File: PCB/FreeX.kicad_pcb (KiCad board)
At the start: 2 copper layers, 2 parts, among them U1 W25Q32JVZPIQ, U3 ESP32-D0WDQ6

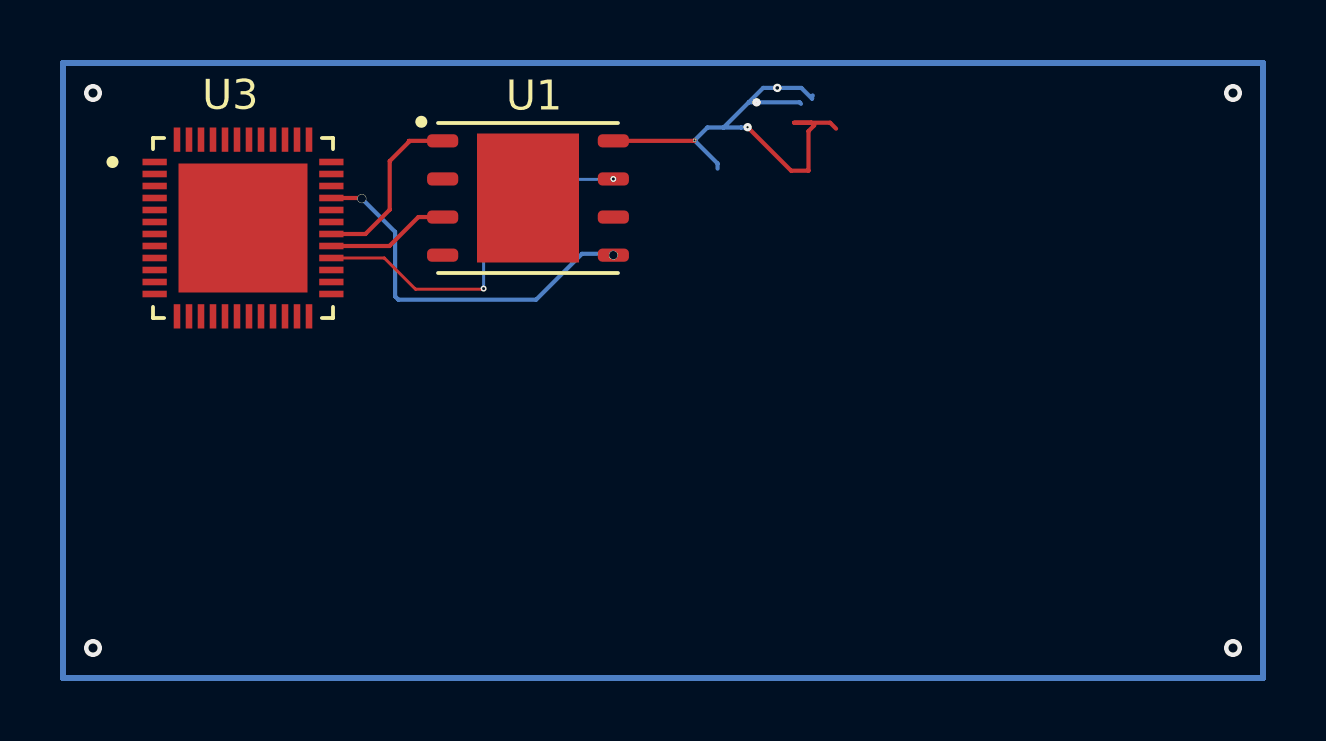
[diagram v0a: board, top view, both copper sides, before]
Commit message: 9th, March 2025
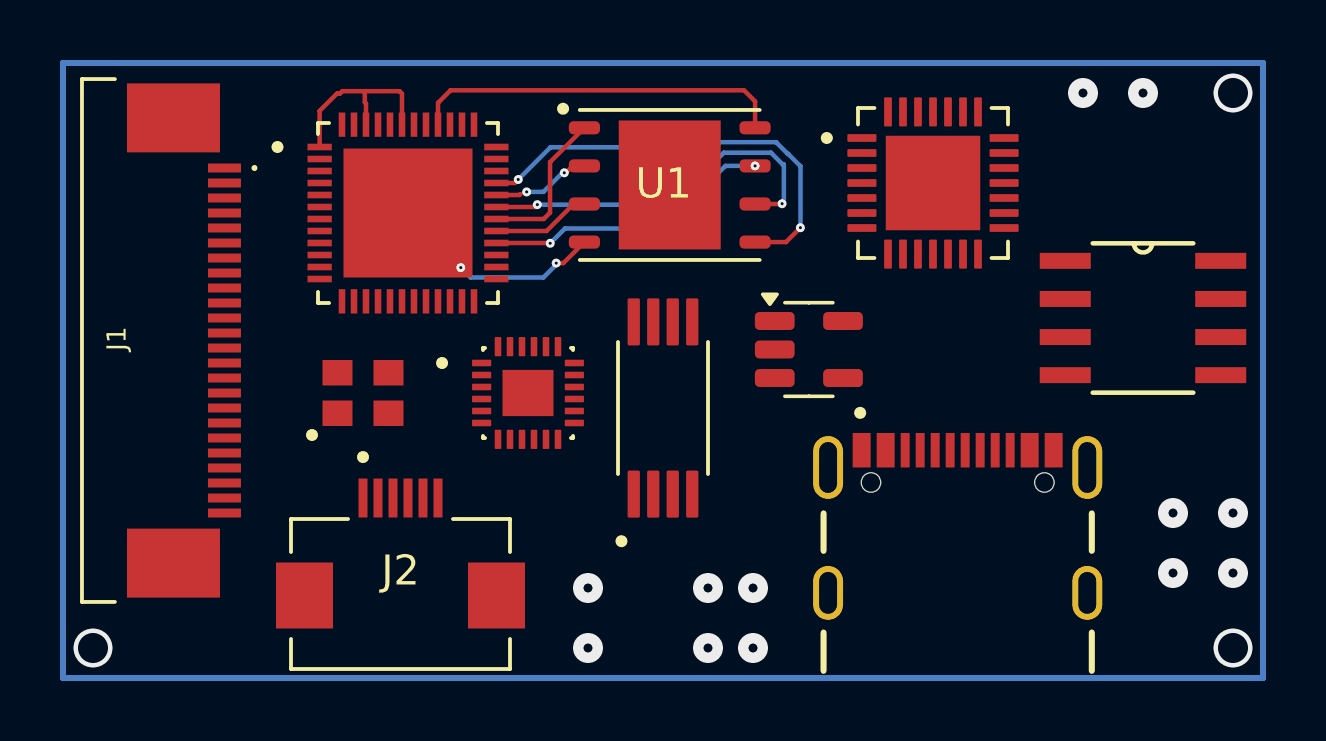
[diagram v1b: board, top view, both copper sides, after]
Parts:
- added J1: 2-1734839-4, 2-1734839-4 pin-24:2-1734839-4 pin-24, F.Cu at (116.7, 89.8)
- added J2: TF31-6S-0.5SH_800_, TF31-6S-0.5SH_800-6-pins:TF31-6S-0.5SH_800-6-pins, F.Cu at (124.2, 98.2)
- added J3: USB4105-GF-A, USB4105-GF-A TYPE C:USB4105-GF-A TYPE C, F.Cu at (142.8, 98.2)
- added U2: MPU-9250, MPU-9250 SENSOR:MPU-9250 SENSOR, F.Cu at (128.5, 91.5)
- added U4: CP2102, CP2102_USB-to-Serial:CP2102_USB-to-Serial, F.Cu at (142.0, 84.5)
- added U5: TC2014-3.3VxCTTR, Package_TO_SOT_SMD:SOT-23-5, F.Cu at (137.9, 90.0)
- added U6: LM358PW, LM358PW-Amplifier:LM358PW-Amplifier, F.Cu at (133.0, 92.0)
- added U7: TDA7052AT_N2, TDA7052AT_N2-Amplifier:TDA7052AT_N2-Amplifier, F.Cu at (149.0, 89.0)
- added Y1: WE-SPXO_IQXO-791, STP_831056298-Crystal-Oscillator:STP_831056298-Crystal-Oscillator, F.Cu at (123.0, 91.5)
- moved U3 5.52 mm to (124.5, 85.5)
- moved U1 4.74 mm to (133.2, 84.6)
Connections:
- U1 pad 8: VDD SDIO -> /VDD SDIO
- U3 pad 40: unconnected-(U3-U0RXD-Pad40) -> /VDD SDIO
- U3 pad 49: unconnected-(U3-GND-Pad49) -> GND
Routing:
- net VDD SDIO: track 17.9 -> 0.00 mm, vias 4 -> 0
- net Net-(U1-CLK): track 0.00 -> 12.7 mm, vias 0 -> 2
- net /VDD SDIO: track 0.00 -> 12.5 mm
- net Net-(U3-VDDA-Pad1): track 0.00 -> 6.42 mm
- net GND: track 0.00 -> 4.77 mm, vias 0 -> 2
- net Net-(U1-DO(IO1)): track 0.00 -> 3.11 mm, vias 0 -> 2
- net Net-(U1-~{HOLD}/RESET(IO3)): track 12.0 -> 9.70 mm
- net Net-(U1-DI(IO0)): track 12.7 -> 14.8 mm, vias 2 -> 15
- net Net-(U1-~{CS}): track 6.41 -> 5.18 mm
- net Net-(U1-~{WP}(IO2)): track 4.11 -> 3.31 mm
- net unconnected-(U7-OUT--Pad8): vias 0 -> 1
- net (no net): vias 4 -> 1
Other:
- board text added: "+"
- board text added: "Buzzer L"
- board text added: "Buzzer R"
- board text added: "Distance L"
- board text added: "Distance R"
- board text added: "MIC"
- board text added: "Speaker"

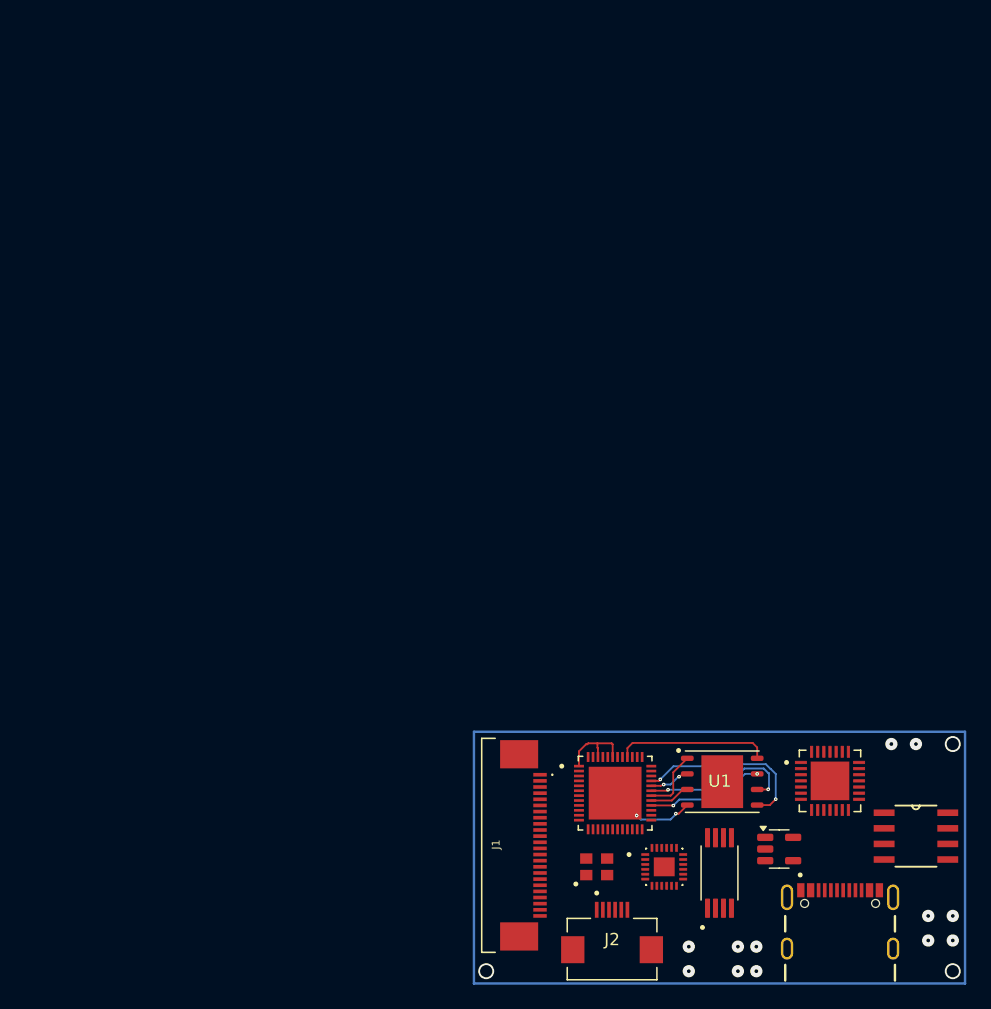
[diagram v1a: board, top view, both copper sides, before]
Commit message: 14th, march. 2025
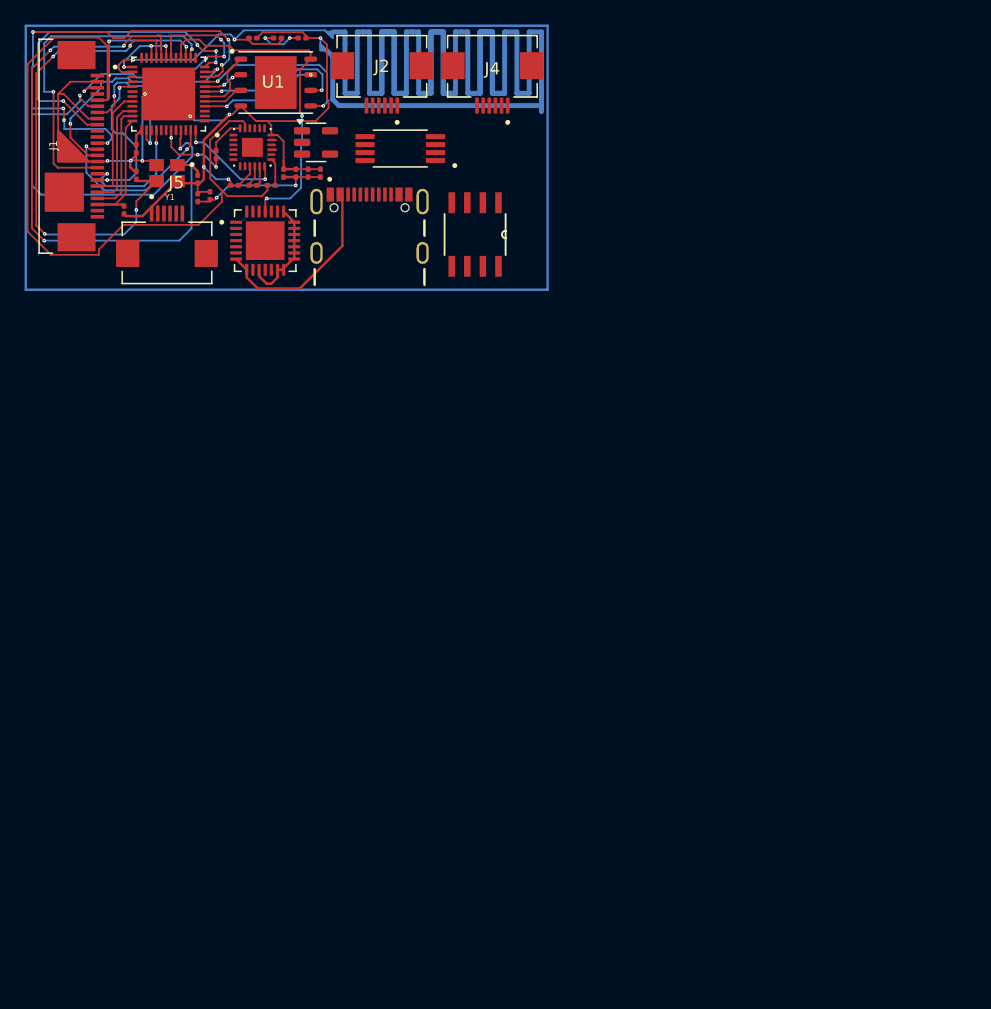
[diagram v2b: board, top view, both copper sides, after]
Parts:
- added C1: 15pf, Capacitor_SMD:C_0201_0603Metric, F.Cu at (85.5, 35.2)
- added C10: 0.1uF, Capacitor_SMD:C_0201_0603Metric, F.Cu at (90.5, 37.0)
- added C11: 0.1uF, Capacitor_SMD:C_0201_0603Metric, F.Cu at (95.0, 36.0)
- added C12: 6.8pF, Capacitor_SMD:C_0201_0603Metric, F.Cu at (97.0, 24.0)
- added C13: 6.8pF, Capacitor_SMD:C_0201_0603Metric, F.Cu at (99.0, 24.0)
- added C2: 15pf, Capacitor_SMD:C_0201_0603Metric, F.Cu at (90.5, 35.5)
- added C3: 12pf, Capacitor_SMD:C_0201_0603Metric, F.Cu at (84.5, 38.0)
- added C4: 12pf, Capacitor_SMD:C_0201_0603Metric, F.Cu at (85.5, 33.0)
- added C5: 10uF, Capacitor_SMD:C_0201_0603Metric, F.Cu at (99.5, 35.0)
- added C6: 0.1uF, Capacitor_SMD:C_0201_0603Metric, F.Cu at (100.5, 35.0)
- added C7: 100pF, Capacitor_SMD:C_0201_0603Metric, F.Cu at (98.5, 35.0)
- added C8: 0.1uF, Capacitor_SMD:C_0201_0603Metric, F.Cu at (97.5, 35.0)
- added C9: 0.1uF, Capacitor_SMD:C_0201_0603Metric, F.Cu at (91.5, 36.8)
- added J4: TF31-6S-0.5SH_800_, TF31-6S-0.5SH_800-6-pins:TF31-6S-0.5SH_800-6-pins, F.Cu at (114.5, 26.3)
- added J5: TF31-6S-0.5SH_800_, TF31-6S-0.5SH_800-6-pins:TF31-6S-0.5SH_800-6-pins, F.Cu at (88.0, 41.5)
- added L1: 1.6nH, Inductor_SMD:L_0201_0603Metric, F.Cu at (95.0, 24.0)
- added R1: 4.7K, Resistor_SMD:R_0201_0603Metric, F.Cu at (92.0, 33.5)
- added R2: 4.7K, Resistor_SMD:R_0201_0603Metric, F.Cu at (96.5, 36.0)
- added R3: 4.7K, Resistor_SMD:R_0201_0603Metric, F.Cu at (93.5, 36.0)
- Y1: value WE-SPXO_IQXO-791 -> ECS-400-10-36-CKY-TR; footprint STP_831056298-Crystal-Oscillator:STP_831056298-Crystal-Oscillator -> 40 MHz_±10ppm_Crystal_10pF_40_Ohms_4-SMD:ECS-400-10-36-CKY-TR
- moved J2 74.3 mm to (105.5, 26.3), turned to 0 degrees
- moved U5 68.8 mm to (100.1, 32.5)
- moved J3 68.4 mm to (104.5, 41.5)
- moved U3 67.6 mm to (88.1, 28.6)
- moved U1 67.6 mm to (96.9, 27.6)
- moved U2 67.5 mm to (95.0, 32.9)
- moved J1 67.4 mm to (80.6, 32.8)
- moved Y1 66.5 mm to (88.0, 35.0), turned to 180 degrees
- moved U6 64.5 mm to (107.0, 33.0), turned to 180 degrees
- moved U4 63.7 mm to (96.0, 40.5)
- moved U7 60.7 mm to (113.1, 40.0), turned to -90 degrees
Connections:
- J1 pad 12: unconnected-(J1-Pad12) -> Net-(U3-GPIO5)
- J1 pad 13: unconnected-(J1-Pad13) -> Net-(U3-GPIO0)
- J1 pad 14: unconnected-(J1-Pad14) -> /D8/GPIO_18
- J1 pad 15: unconnected-(J1-Pad15) -> GND
- J1 pad 16: unconnected-(J1-Pad16) -> /D7/GPIO_19
- J1 pad 17: unconnected-(J1-Pad17) -> /PCLK/GPIO_27
- J1 pad 18: unconnected-(J1-Pad18) -> Net-(U3-SENSOR_VP)
- J1 pad 19: unconnected-(J1-Pad19) -> Net-(U3-SENSOR_VN)
- J1 pad 2: unconnected-(J1-Pad2) -> GND
- J1 pad 20: unconnected-(J1-Pad20) -> Net-(U3-VDET_1)
- J1 pad 21: unconnected-(J1-Pad21) -> Net-(U3-VDET_2)
- J1 pad 22: unconnected-(J1-Pad22) -> /D4/32K_XP/GPIO_32
- J1 pad 3: unconnected-(J1-Pad3) -> Net-(U3-GPIO21)
- J1 pad 5: unconnected-(J1-Pad5) -> /SCL/GPIO_22
- J1 pad 6: unconnected-(J1-Pad6) -> /RESET/MTDO/GPIO 15
- J1 pad 7: unconnected-(J1-Pad7) -> /VS/GPIO_25
- J1 pad 8: unconnected-(J1-Pad8) -> GND
- J1 pad 9: unconnected-(J1-Pad9) -> /HS/GPIO_23
- J1 pad SH1: Net-(J1-SHIELD-PadSH1) -> unconnected-(J1-SHIELD-PadSH1)_0
- J1 pad SH2: Net-(J1-SHIELD-PadSH1) -> unconnected-(J1-SHIELD-PadSH1)
- J3 pad A1_B12: Net-(J3-GND-PadA1_B12) -> GND
- J3 pad A4_B9: Net-(J3-VBUS-PadA4_B9) -> Net-(U4-REGIN)
- J3 pad B1_A12: Net-(J3-GND-PadA1_B12) -> GND
- J3 pad B4_A9: Net-(J3-VBUS-PadA4_B9) -> Net-(U4-REGIN)
- J3 pad B6: unconnected-(J3-DP2-PadB6) -> Net-(J3-DP2)
- J3 pad B7: unconnected-(J3-DN2-PadB7) -> Net-(J3-DN2)
- U1 pad 8: /VDD SDIO -> /PROG_RXD
- U2 pad 10: unconnected-(U2-REGOUT-Pad10) -> Net-(U2-REGOUT)
- U2 pad 11: unconnected-(U2-FSYNC-Pad11) -> GND
- U2 pad 12: unconnected-(U2-INT-Pad12) -> /INT/GPIO_4
- U2 pad 13: unconnected-(U2-VDD-Pad13) -> /VDD33
- U2 pad 18: unconnected-(U2-GND-Pad18) -> GND
- U2 pad 23: unconnected-(U2-SCL/SCLK-Pad23) -> /SCL/GPIO_22
- U2 pad 24: unconnected-(U2-SDA/SDI-Pad24) -> /SDA/GPIO_21
- U2 pad 9: unconnected-(U2-AD0/SDO-Pad9) -> Net-(U2-AD0/SDO)
- U3 pad 1: Net-(U3-VDDA-Pad1) -> /VCC3.3V
- U3 pad 10: unconnected-(U3-VDET_1-Pad10) -> Net-(U3-VDET_1)
- U3 pad 11: unconnected-(U3-VDET_2-Pad11) -> Net-(U3-VDET_2)
- U3 pad 12: unconnected-(U3-32K_XP-Pad12) -> /D4/32K_XP/GPIO_32
- U3 pad 13: unconnected-(U3-32K_XN-Pad13) -> Net-(U3-32K_XN)
- U3 pad 14: unconnected-(U3-GPIO25-Pad14) -> /VS/GPIO_25
- U3 pad 16: unconnected-(U3-GPIO27-Pad16) -> /PCLK/GPIO_27
- U3 pad 19: unconnected-(U3-VDD3P3_RTC-Pad19) -> /VCC3.3V
- U3 pad 2: unconnected-(U3-LNA_IN-Pad2) -> /ANTENNA
- U3 pad 21: unconnected-(U3-MTDO-Pad21) -> /RESET/MTDO/GPIO 15
- U3 pad 22: unconnected-(U3-GPIO2-Pad22) -> /VDD 3.3V POWER
- U3 pad 23: unconnected-(U3-GPIO0-Pad23) -> Net-(U3-GPIO0)
- U3 pad 24: unconnected-(U3-GPIO4-Pad24) -> /INT/GPIO_4
- U3 pad 3: Net-(U3-VDD3P3-Pad3) -> /VCC3.3V
- U3 pad 34: unconnected-(U3-GPIO5-Pad34) -> Net-(U3-GPIO5)
- U3 pad 35: unconnected-(U3-GPIO18-Pad35) -> /D8/GPIO_18
- U3 pad 36: unconnected-(U3-GPIO23-Pad36) -> /HS/GPIO_23
- U3 pad 37: unconnected-(U3-VDD3P3_CPU-Pad37) -> /VCC3.3V
- U3 pad 38: unconnected-(U3-GPIO19-Pad38) -> /D7/GPIO_19
- U3 pad 39: unconnected-(U3-GPIO22-Pad39) -> /SCL/GPIO_22
- U3 pad 4: Net-(U3-VDD3P3-Pad3) -> /VCC3.3V
- U3 pad 40: /VDD SDIO -> /PROG_RXD
- U3 pad 41: unconnected-(U3-U0TXD-Pad41) -> /PROG_TXD
- U3 pad 42: unconnected-(U3-GPIO21-Pad42) -> Net-(U3-GPIO21)
- U3 pad 43: Net-(U3-VDDA-Pad1) -> /VCC3.3V
- U3 pad 44: unconnected-(U3-XTAL_N-Pad44) -> Net-(U3-XTAL_N)
- U3 pad 45: unconnected-(U3-XTAL_P-Pad45) -> Net-(U3-XTAL_P)
- U3 pad 46: Net-(U3-VDDA-Pad1) -> /VCC3.3V
- U3 pad 5: unconnected-(U3-SENSOR_VP-Pad5) -> Net-(U3-SENSOR_VP)
- U3 pad 8: unconnected-(U3-SENSOR_VN-Pad8) -> Net-(U3-SENSOR_VN)
- U4 pad 25: unconnected-(U4-RXD-Pad25) -> /PROG_RXD
- U4 pad 26: unconnected-(U4-TXD-Pad26) -> /PROG_TXD
- U4 pad 4: unconnected-(U4-D+-Pad4) -> Net-(J3-DP2)
- U4 pad 5: unconnected-(U4-D--Pad5) -> Net-(J3-DN2)
- U4 pad 7: unconnected-(U4-REGIN-Pad7) -> Net-(U4-REGIN)
- U4 pad 8: unconnected-(U4-VBUS-Pad8) -> Net-(U4-REGIN)
- Y1 pad 1: unconnected-(Y1-E/D-Pad1) -> Net-(U3-XTAL_N)
- Y1 pad 2: unconnected-(Y1-GND-Pad2) -> GND
- Y1 pad 3: unconnected-(Y1-OUT-Pad3) -> Net-(U3-XTAL_P)
- Y1 pad 4: unconnected-(Y1-+VS-Pad4) -> GND
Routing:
- net /ANTENNA: track 0.00 -> 186.0 mm, vias 0 -> 2
- net GND: track 4.77 -> 82.1 mm, vias 2 -> 9
- net /SCL/GPIO_22: track 0.00 -> 72.1 mm, vias 0 -> 2
- net Net-(U3-XTAL_N): track 0.00 -> 47.7 mm, vias 0 -> 4
- net Net-(U3-XTAL_P): track 0.00 -> 39.4 mm, vias 0 -> 4
- net Net-(U3-GPIO5): track 0.00 -> 37.8 mm, vias 0 -> 6
- net /RESET/MTDO/GPIO 15: track 0.00 -> 30.7 mm, vias 0 -> 2
- net /PROG_RXD: track 0.00 -> 28.0 mm, vias 0 -> 2
- net /D7/GPIO_19: track 0.00 -> 28.0 mm, vias 0 -> 2
- net /HS/GPIO_23: track 0.00 -> 27.8 mm, vias 0 -> 4
- net Net-(U3-GPIO21): track 0.00 -> 21.5 mm, vias 0 -> 4
- net /D8/GPIO_18: track 0.00 -> 19.6 mm, vias 0 -> 2
- net /VCC3.3V: track 0.00 -> 19.3 mm, vias 0 -> 5
- net Net-(U4-REGIN): track 0.00 -> 15.7 mm
- net Net-(U3-GPIO0): track 0.00 -> 15.0 mm, vias 0 -> 2
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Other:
- board text removed: "+"
- board text removed: "Buzzer L"
- board text removed: "Buzzer R"
- board text removed: "Distance L"
- board text removed: "Distance R"
- board text removed: "MIC"
- board text removed: "Speaker"
